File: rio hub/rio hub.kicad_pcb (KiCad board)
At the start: 2 copper layers, 160.8 x 155.2 mm, 1 part

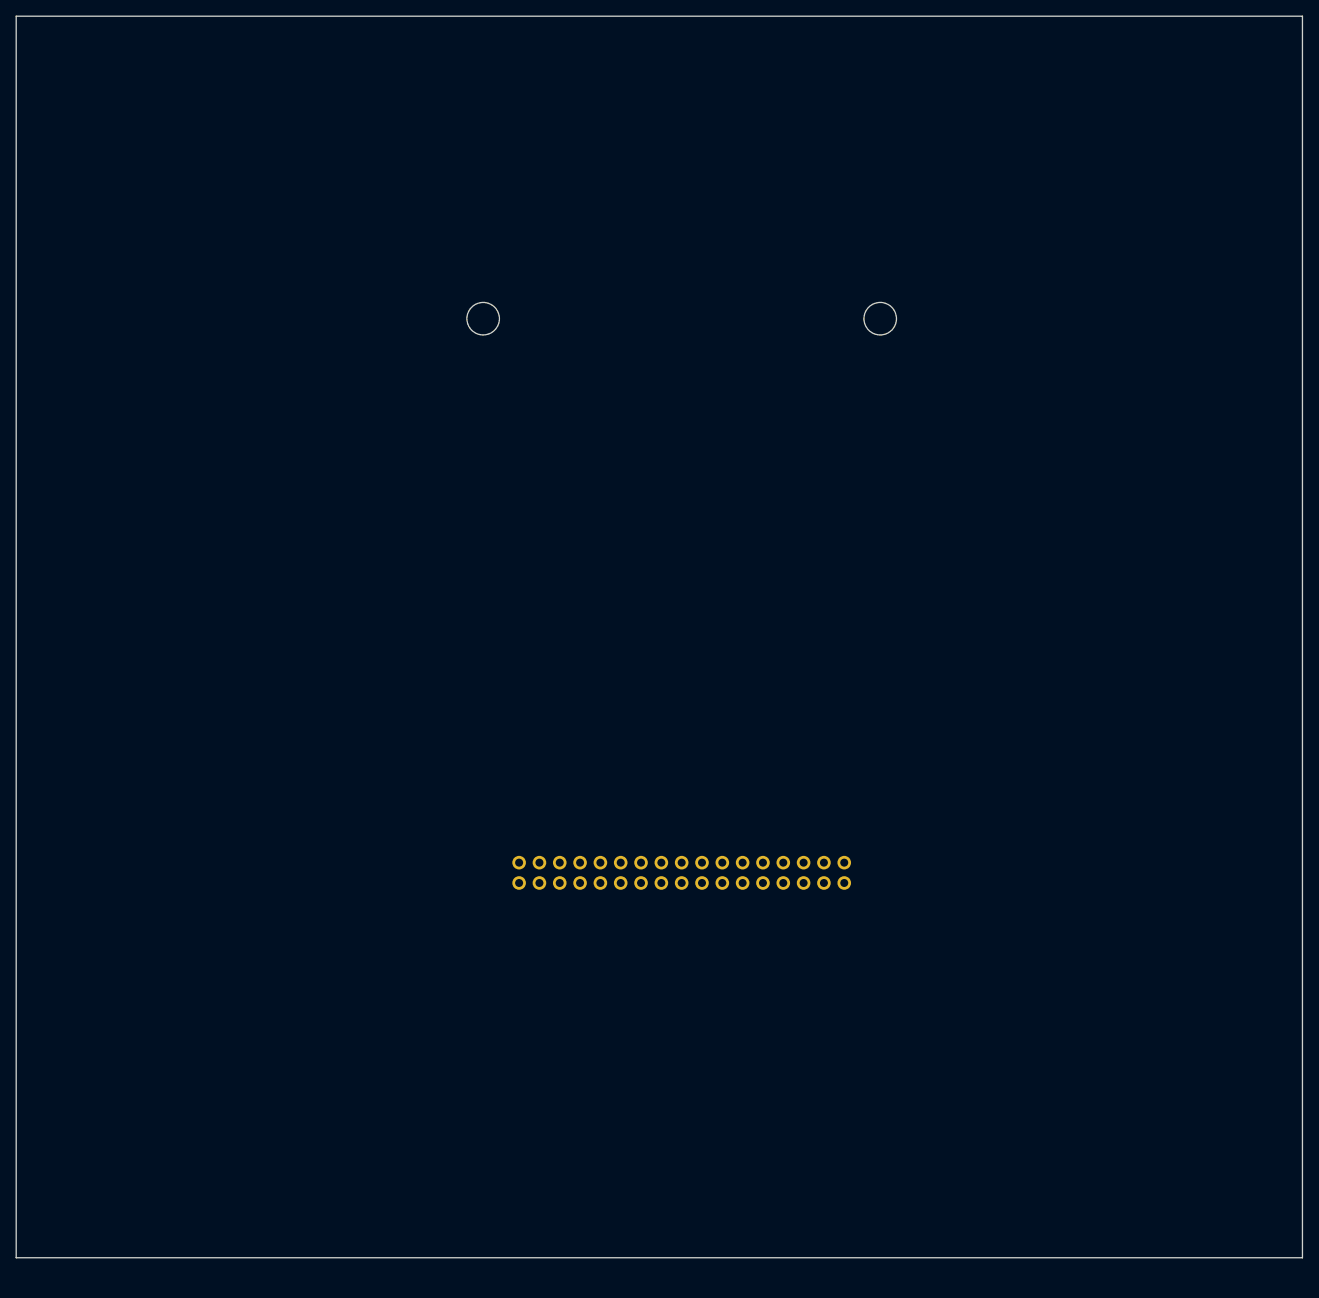
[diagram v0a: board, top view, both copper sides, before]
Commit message: fixed diode placement, major rio hub work
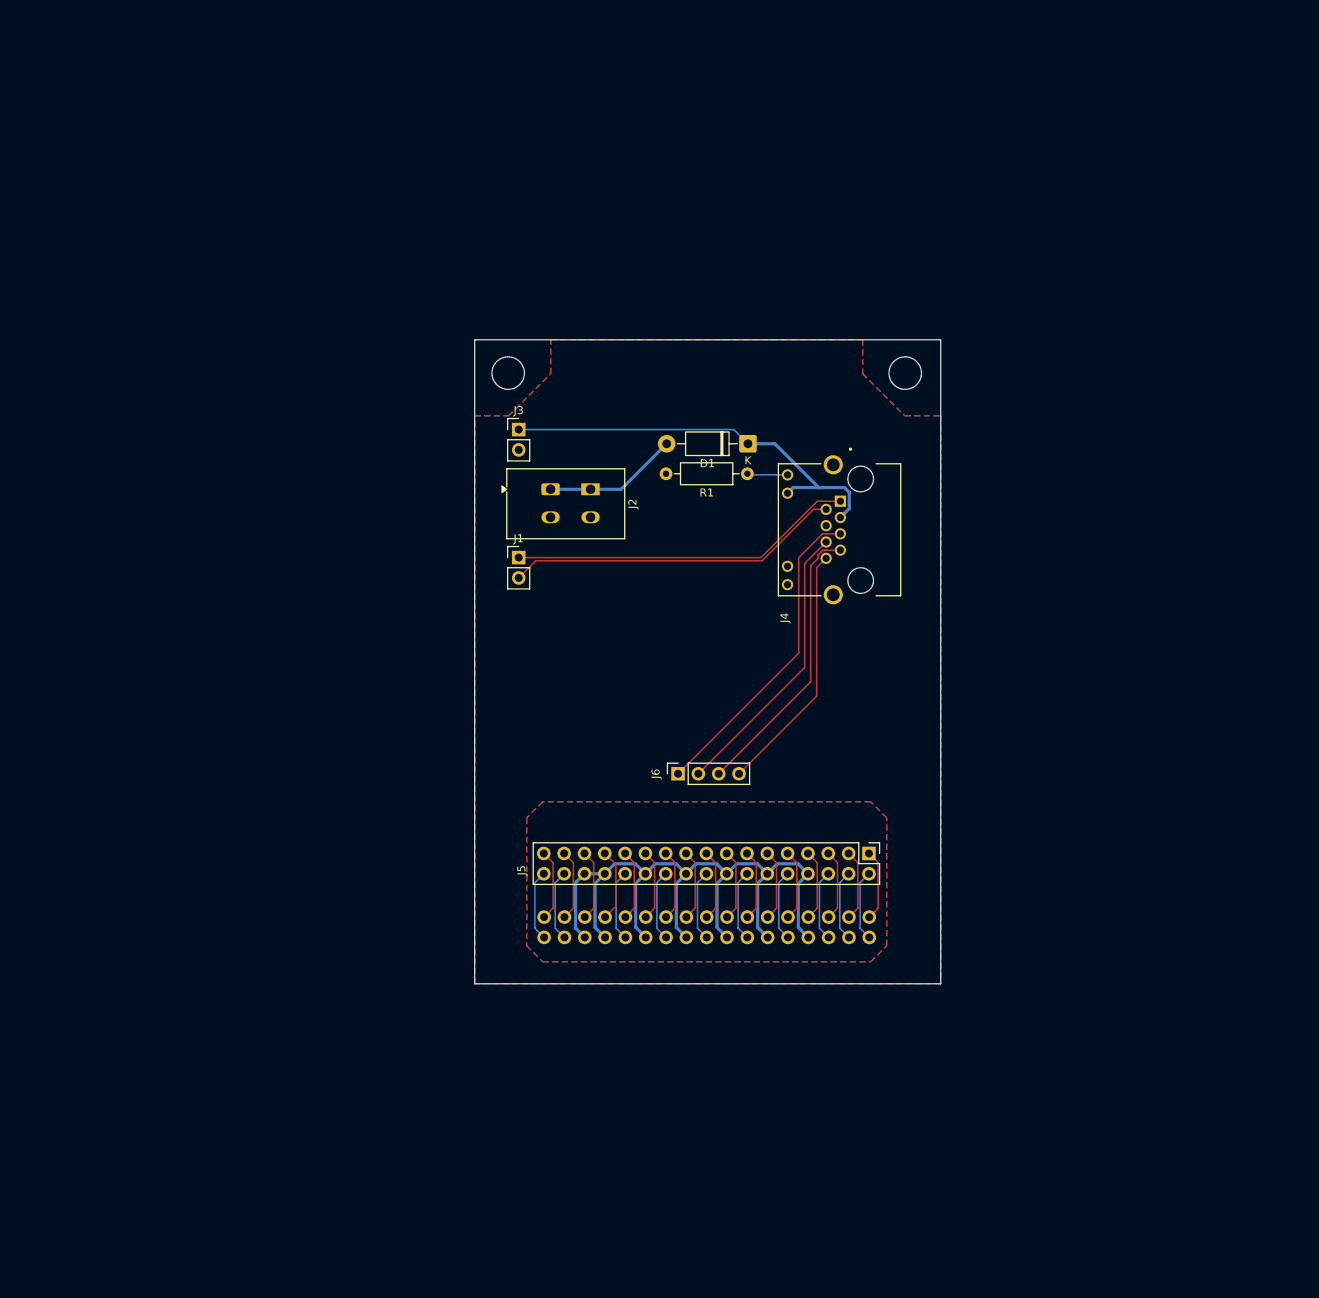
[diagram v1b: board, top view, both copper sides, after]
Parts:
- added D1: D_Schottky, Diode_THT:D_DO-41_SOD81_P10.16mm_Horizontal, F.Cu at (135.2, 72.8)
- added J1: Conn_01x02_Pin, Connector_PinHeader_2.54mm:PinHeader_1x02_P2.54mm_Vertical, F.Cu at (106.5, 87.0)
- added J2: Conn_01x02_Pin, TerminalBlock_WAGO:TerminalBlock_WAGO_2601-1102_1x02_P3.50mm_Horizontal, F.Cu at (110.5, 78.4)
- added J3: Conn_01x02_Pin, Connector_PinHeader_2.54mm:PinHeader_1x02_P2.54mm_Vertical, F.Cu at (106.5, 71.0)
- added J4: MTJ-88ARX1-FSM-LG, custom:ADAMTECH_MTJ-88ARX1-FSM-LG, F.Cu at (149.2, 83.5)
- added J5: Conn_02x17_Odd_Even, Connector_PinSocket_2.54mm:PinSocket_2x17_P2.54mm_Vertical, F.Cu at (150.3, 127.3)
- added J6: Conn_01x04_Socket, Connector_PinSocket_2.54mm:PinSocket_1x04_P2.54mm_Vertical, F.Cu at (126.4, 114.0)
- added R1: R, Resistor_THT:R_Axial_DIN0207_L6.3mm_D2.5mm_P10.16mm_Horizontal, F.Cu at (135.1, 76.5)
- U1: footprint FRC:RoboRIO-THT -> FRC:RoboRIO_MXP-THT
- moved U1 7.49 mm to (105.2, 63.9)
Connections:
- U1 pad 1: unconnected-(U1I-MXP_5V-Pad1) -> Net-(J5-Pin_1)
- U1 pad 10: unconnected-(U1I-MXP_RX-Pad10) -> Net-(J5-Pin_10)
- U1 pad 11: unconnected-(U1I-MXP_DIO0_PWM0-Pad11) -> Net-(J5-Pin_11)
- U1 pad 12: unconnected-(U1I-MXP_DGND-Pad12) -> /DGND
- U1 pad 13: unconnected-(U1I-MXP_DIO1_PWM1-Pad13) -> Net-(J5-Pin_13)
- U1 pad 14: unconnected-(U1I-MXP_TX-Pad14) -> Net-(J5-Pin_14)
- U1 pad 15: unconnected-(U1I-MXP_DIO2_PWM2-Pad15) -> Net-(J5-Pin_15)
- U1 pad 16: unconnected-(U1I-MXP_DGND-Pad16) -> /DGND
- U1 pad 17: unconnected-(U1I-MXP_DIO3_PWM3-Pad17) -> Net-(J5-Pin_17)
- U1 pad 18: unconnected-(U1I-MXP_DIO11_PWM7-Pad18) -> Net-(J5-Pin_18)
- U1 pad 19: unconnected-(U1I-MXP_DIO4_CS-Pad19) -> Net-(J5-Pin_19)
- U1 pad 2: unconnected-(U1I-MXP_AO0-Pad2) -> Net-(J5-Pin_2)
- U1 pad 20: unconnected-(U1I-MXP_DGND-Pad20) -> /DGND
- U1 pad 21: unconnected-(U1I-MXP_DIO5_SCLK-Pad21) -> Net-(J5-Pin_21)
- U1 pad 22: unconnected-(U1I-MXP_DIO12_PWM8-Pad22) -> Net-(J5-Pin_22)
- U1 pad 23: unconnected-(U1I-MXP_DIO6_MISO-Pad23) -> Net-(J5-Pin_23)
- U1 pad 24: unconnected-(U1I-MXP_DGND-Pad24) -> /DGND
- U1 pad 25: unconnected-(U1I-MXP_DIO7_MOSI-Pad25) -> Net-(J5-Pin_25)
- U1 pad 26: unconnected-(U1I-MXP_DIO13_PWM9-Pad26) -> Net-(J5-Pin_26)
- U1 pad 27: unconnected-(U1I-MXP_DIO8_PWM4-Pad27) -> Net-(J5-Pin_27)
- U1 pad 28: unconnected-(U1I-MXP_DGND-Pad28) -> /DGND
- U1 pad 29: unconnected-(U1I-MXP_DIO9_PWM5-Pad29) -> Net-(J5-Pin_29)
- U1 pad 3: unconnected-(U1I-MXP_AI0-Pad3) -> Net-(J5-Pin_3)
- U1 pad 30: unconnected-(U1I-MXP_DGND-Pad30) -> /DGND
- U1 pad 31: unconnected-(U1I-MXP_DIO10_PWM6-Pad31) -> Net-(J5-Pin_31)
- U1 pad 32: unconnected-(U1I-MXP_DIO14_SCL-Pad32) -> Net-(J5-Pin_32)
- U1 pad 33: unconnected-(U1I-MXP_3V3-Pad33) -> Net-(J5-Pin_33)
- U1 pad 34: unconnected-(U1I-MXP_DIO15_SDA-Pad34) -> Net-(J5-Pin_34)
- U1 pad 4: unconnected-(U1I-MXP_AO1-Pad4) -> Net-(J5-Pin_4)
- U1 pad 5: unconnected-(U1I-MXP_AI1-Pad5) -> Net-(J5-Pin_5)
- U1 pad 6: unconnected-(U1I-MXP_AGND-Pad6) -> /AGND
- U1 pad 7: unconnected-(U1I-MXP_AI2-Pad7) -> Net-(J5-Pin_7)
- U1 pad 8: unconnected-(U1I-MXP_DGND-Pad8) -> /DGND
- U1 pad 9: unconnected-(U1I-MXP_AI3-Pad9) -> Net-(J5-Pin_9)
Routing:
- net /DGND: track 0.00 -> 95.9 mm
- net /12v: track 0.00 -> 52.4 mm
- net Net-(J1-Pin_1): track 0.00 -> 43.1 mm
- net Net-(J1-Pin_2): track 0.00 -> 42.0 mm
- net Net-(J6-Pin_1): track 0.00 -> 39.7 mm
- net Net-(J6-Pin_2): track 0.00 -> 35.6 mm
- net Net-(J6-Pin_3): track 0.00 -> 35.5 mm
- net Net-(J6-Pin_4): track 0.00 -> 31.4 mm
- net Net-(D1-A): track 0.00 -> 16.9 mm
- net Net-(J5-Pin_27): track 0.00 -> 9.09 mm
- net Net-(J5-Pin_4): track 0.00 -> 8.89 mm
- net Net-(J5-Pin_18): track 0.00 -> 8.89 mm
- net Net-(J5-Pin_10): track 0.00 -> 8.89 mm
- net Net-(J5-Pin_7): track 0.00 -> 8.89 mm
- net Net-(J5-Pin_34): track 0.00 -> 8.89 mm
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- added copper zone on B.Cu, net /DGND
- added copper zone on F.Cu, net /DGND
- added copper zone on B.Cu, net /GND
- added copper zone on F.Cu, net /GND
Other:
- board size 160.8 x 155.2 mm -> 58.2 x 80.5 mm

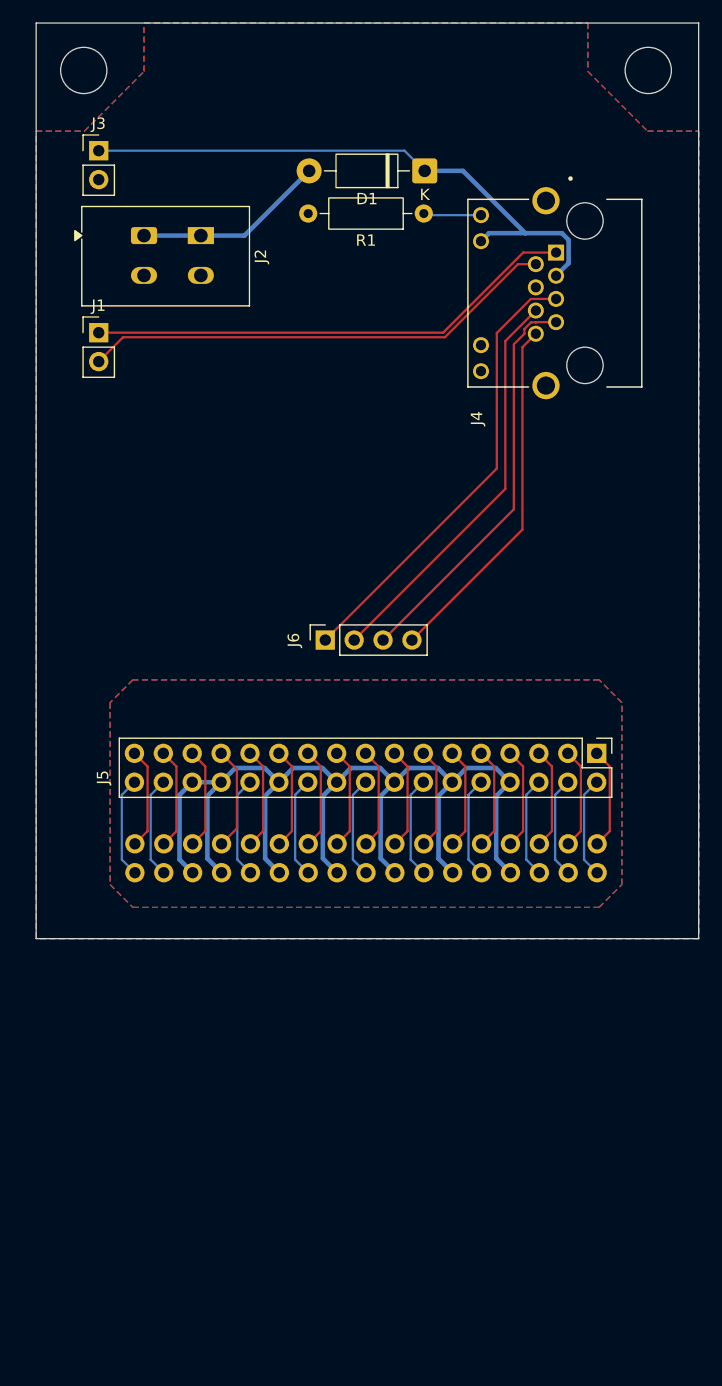
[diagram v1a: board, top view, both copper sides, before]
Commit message: rio hub work
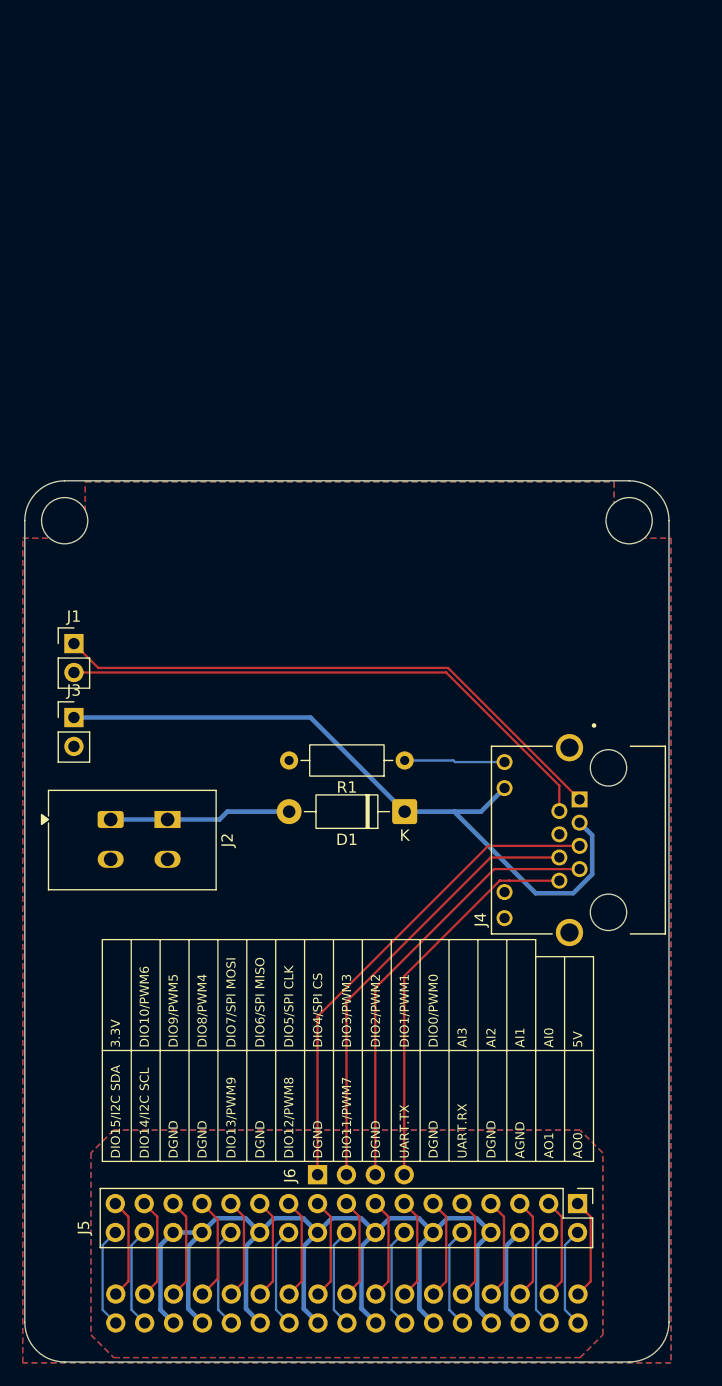
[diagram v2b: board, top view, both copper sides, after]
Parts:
- moved D1 56.4 mm to (133.4, 129.1)
- moved J2 51.4 mm to (107.6, 129.8)
- moved J3 49.9 mm to (104.3, 120.8)
- moved J4 48.1 mm to (151.3, 131.6)
- moved R1 48.1 mm to (133.4, 124.6)
- moved J6 47.0 mm to (125.7, 161.0)
- moved U1 39.6 mm to (103.5, 103.5)
- moved J5 39.6 mm to (148.6, 166.9)
- moved J1 27.4 mm to (104.3, 114.3)
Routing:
- net /12v: track 52.4 -> 62.9 mm
- net Net-(J1-Pin_2): track 42.0 -> 49.0 mm
- net Net-(J1-Pin_1): track 43.1 -> 50.1 mm
- net Net-(J4-Pad9): track 5.09 -> 8.84 mm
- net Net-(J6-Pin_2): track 35.6 -> 39.2 mm
- net Net-(J6-Pin_1): track 39.7 -> 43.2 mm
- net Net-(J6-Pin_3): track 35.5 -> 38.7 mm
- net Net-(J6-Pin_4): track 31.4 -> 34.6 mm
- net Net-(D1-A): track 16.9 -> 16.0 mm
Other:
- board size 58.2 x 80.5 mm -> 56.6 x 77.5 mm
- board text added: "3.3V"
- board text added: "5V"
- board text added: "AGND"
- board text added: "AI0"
- board text added: "AI1"
- board text added: "AI2"
- board text added: "AI3"
- board text added: "AO0"
- board text added: "AO1"
- board text added: "DGND"
- board text added: "DIO0/PWM0"
- board text added: "DIO1/PWM1"
- board text added: "DIO10/PWM6"
- board text added: "DIO11/PWM7"
- board text added: "DIO12/PWM8"
- board text added: "DIO13/PWM9"
- board text added: "DIO14/I2C SCL"
- board text added: "DIO15/I2C SDA"
- board text added: "DIO2/PWM2"
- board text added: "DIO3/PWM3"
- board text added: "DIO4/SPI CS"
- board text added: "DIO5/SPI CLK"
- board text added: "DIO6/SPI MISO"
- board text added: "DIO7/SPI MOSI"
- board text added: "DIO8/PWM4"
- board text added: "DIO9/PWM5"
- board text added: "UART.RX"
- board text added: "UART.TX"
